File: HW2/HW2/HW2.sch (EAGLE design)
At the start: 1 part

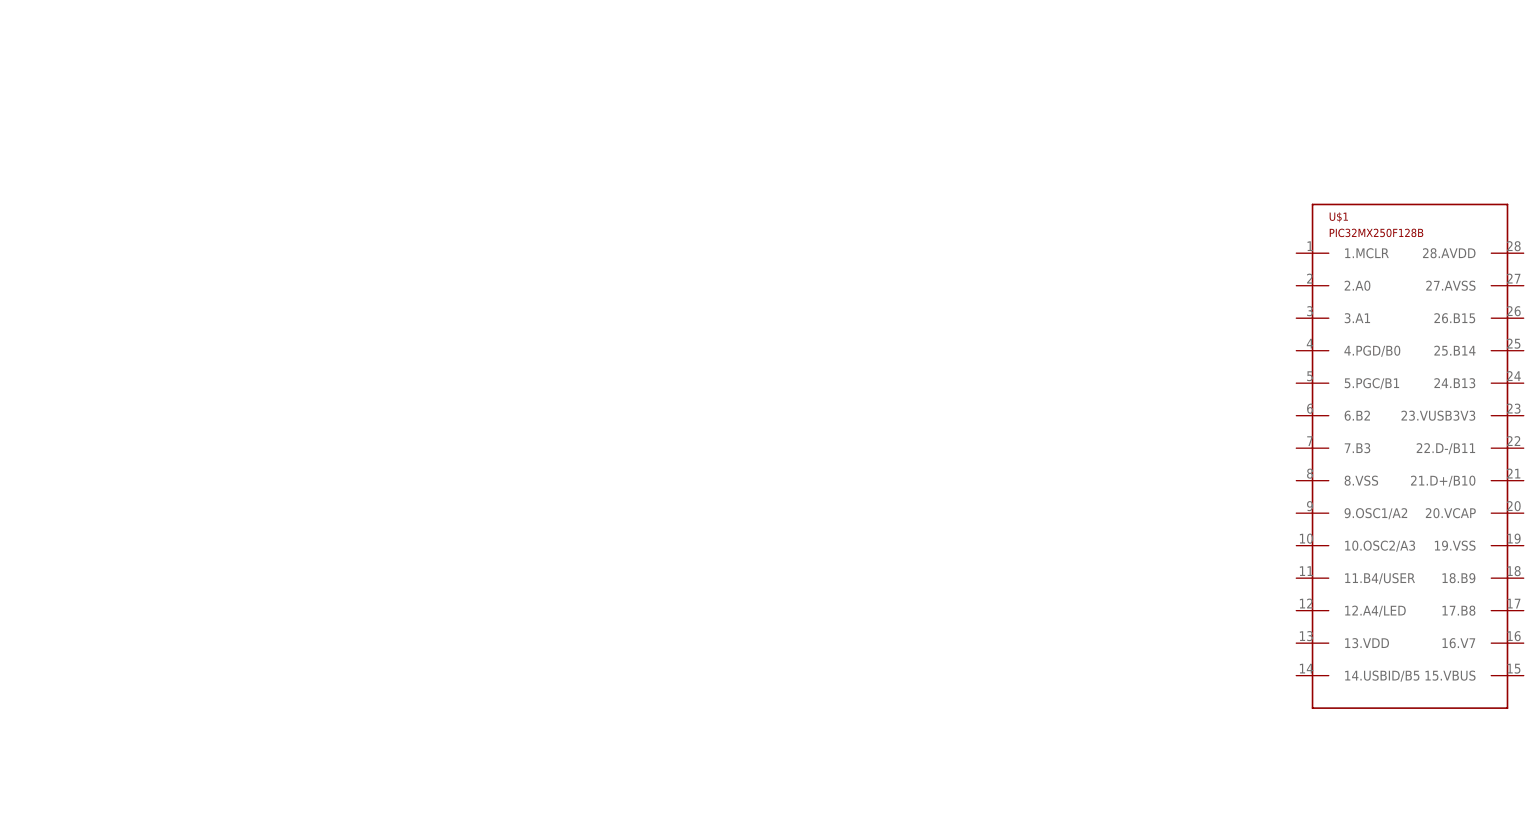
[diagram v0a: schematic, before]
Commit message: Finish Schematic
HW2 complete
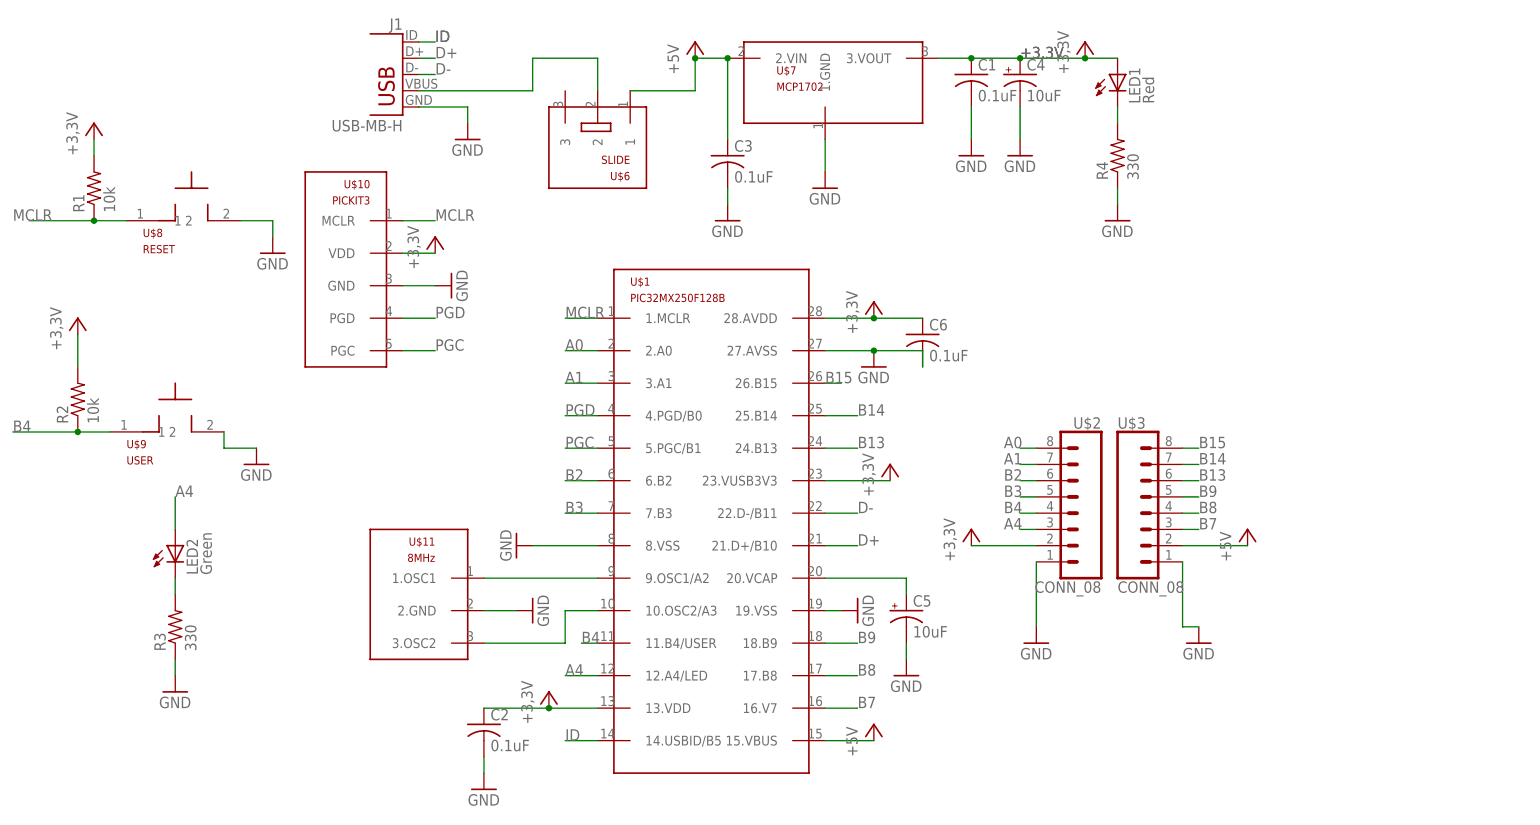
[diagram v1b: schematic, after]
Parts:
- added C1, C2, C3, C6: 0.1uF, HW2:C-US025-025X050
- added C4, C5: 10uF, HW2:CPOL-USB45181B
- added J1: USB-MB-H, HW2:USB-MB-H
- added LED1: Red, led:LED3MM
- added LED2: Green, led:LED3MM
- added R1, R2: 10k, HW2:R-US_0207/10
- added R3, R4: 330, HW2:R-US_0207/10
- added U$10: PICKIT3, HW2:PICKIT3
- added U$11: 8MHz, HW2:OSC
- added U$2, U$3: CONN_08, HW2:CONN_08
- added U$6: SLIDE, HW2:SLIDE
- added U$7: MCP1702, HW2:MCP1702
- added U$8: RESET, HW2:PB
- added U$9: USER, HW2:PB
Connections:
- new net +3,3V: C1.1, C2.1, C4.+, C6.1, LED1.A, R1.2, R2.2, U$1.13.VDD, U$1.23.VUSB3V3, U$1.28.AVDD, U$10.VDD, U$2.2, U$7.3.VOUT
- new net +5V: C3.1, U$1.15.VBUS, U$3.2, U$6.1, U$7.2.VIN
- new net A0: U$1.2.A0, U$2.8
- new net A1: U$1.3.A1, U$2.7
- new net A4: LED2.A, U$1.12.A4/LED, U$2.3
- new net B13: U$1.24.B13, U$3.6
- new net B14: U$1.25.B14, U$3.7
- new net B15: U$1.26.B15, U$3.8
- new net B2: U$1.6.B2, U$2.6
- new net B3: U$1.7.B3, U$2.5
- new net B4: R2.1, U$1.11.B4/USER, U$2.4, U$9.1
- new net B7: U$1.16.V7, U$3.3
- new net B8: U$1.17.B8, U$3.4
- new net B9: U$1.18.B9, U$3.5
- new net D+: J1.D+, U$1.21.D+/B10
- new net D-: J1.D-, U$1.22.D-/B11
- new net GND: C1.2, C2.2, C3.2, C4.-, C5.-, C6.2, J1.GND, R3.1, R4.1, U$1.19.VSS, U$1.27.AVSS, U$1.8.VSS, U$10.GND, U$11.2.GND, U$2.1, U$3.1, U$7.1.GND, U$8.2, U$9.2
- new net ID: J1.ID, U$1.14.USBID/B5
- new net MCLR: R1.1, U$1.1.MCLR, U$10.MCLR, U$8.1
- new net N$1: J1.VBUS, U$6.2
- new net N$2: LED1.C, R4.2
- new net N$3: U$1.9.OSC1/A2, U$11.1.OSC1
- new net N$4: U$1.10.OSC2/A3, U$11.3.OSC2
- new net N$5: C5.+, U$1.20.VCAP
- new net N$6: LED2.C, R3.2
- new net PGC: U$1.5.PGC/B1, U$10.PGC
- new net PGD: U$1.4.PGD/B0, U$10.PGD
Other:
- moved on the sheet: U$1
